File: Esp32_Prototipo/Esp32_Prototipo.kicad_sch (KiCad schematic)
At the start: 18 parts, among them J1 Fan, J2 Screw_Terminal_01x04, J3 Screw_Terminal_01x04, J4 Input, Q1 2N7002K, U1 ESP32-DEVKITC-32D

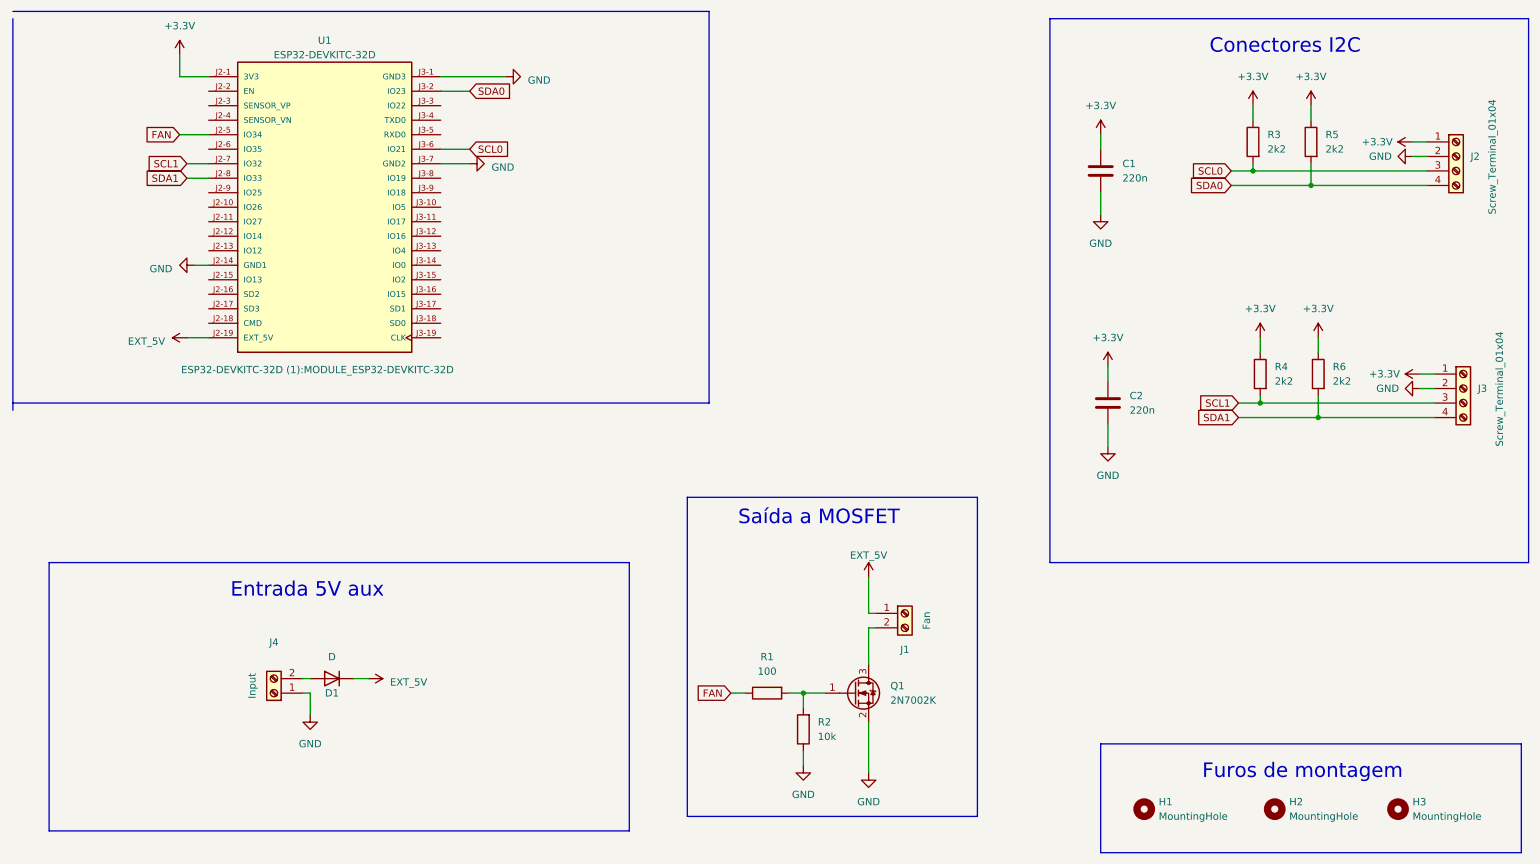
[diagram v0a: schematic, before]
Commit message: proto esp32 pronto para montar
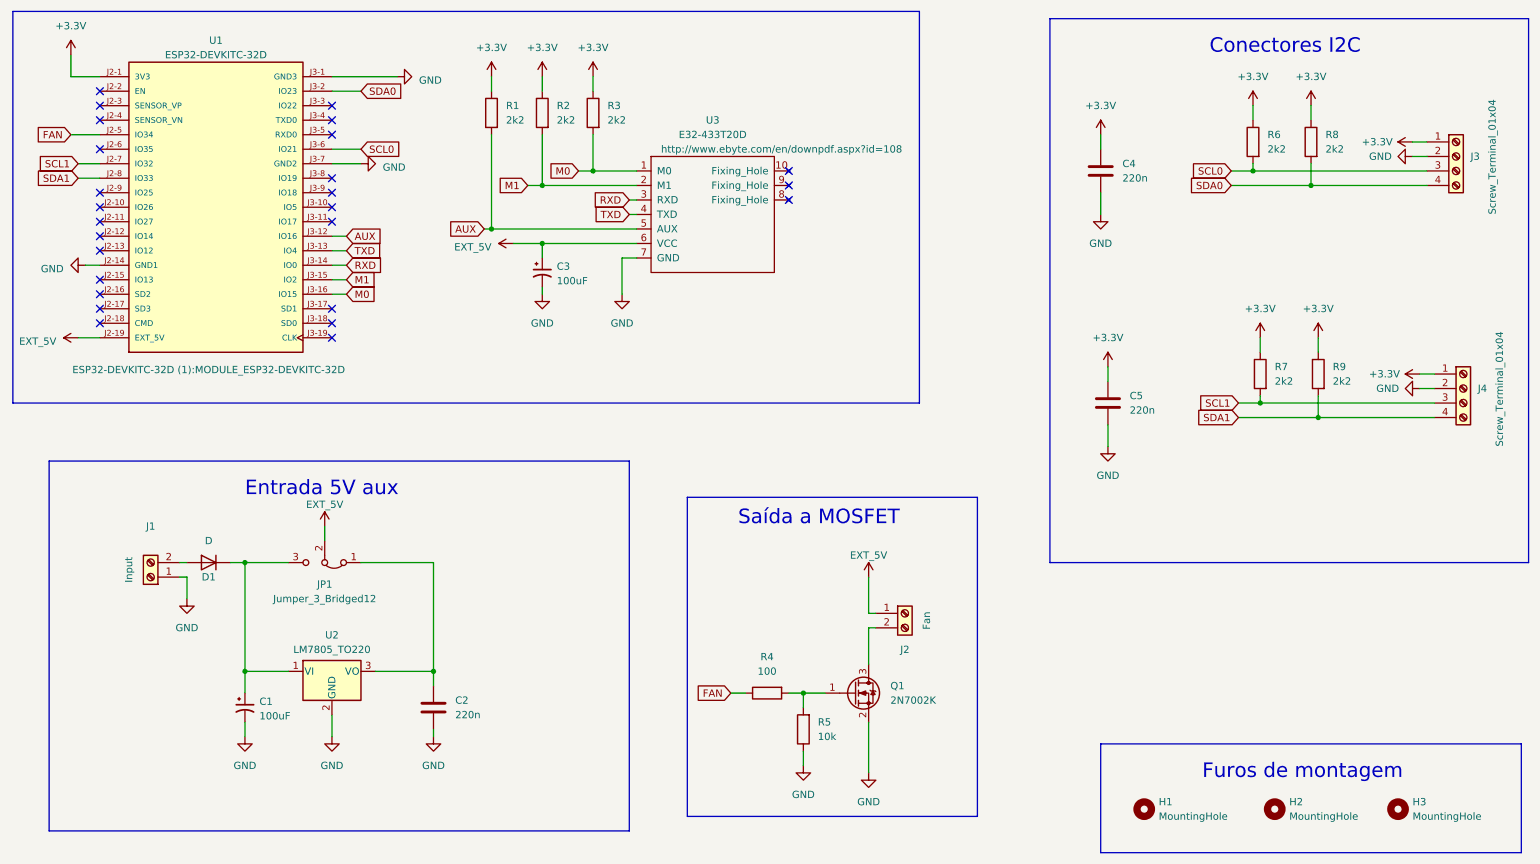
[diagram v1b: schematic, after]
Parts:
- added C1, C3: 100uF, Capacitor_THT:CP_Radial_D6.3mm_P2.50mm, symbol Device:C_Polarized_Small_US
- added C2: 220n, Capacitor_THT:C_Disc_D5.0mm_W2.5mm_P5.00mm, symbol Device:C
- added JP1: Jumper_3_Bridged12, Connector_PinHeader_2.54mm:PinHeader_1x03_P2.54mm_Vertical, symbol Jumper:Jumper_3_Bridged12
- added R1, R2, R3: 2k2, Resistor_THT:R_Axial_DIN0207_L6.3mm_D2.5mm_P10.16mm_Horizontal, symbol Device:R
- added U2: LM7805_TO220, Package_TO_SOT_THT:TO-220-3_Vertical, symbol Regulator_Linear:LM7805_TO220
- added U3: E32-433T20D, footprints6:E32-xxxT20D, symbol E32-xxxT20D:E32-433T20D
- renumbered C1 to C4, C2 to C5, J4 to J1, J1 to J2, J2 to J3, J3 to J4, R1 to R4, R2 to R5, R3 to R6, R4 to R7, R5 to R8, R6 to R9
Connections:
- net +3V3: now also R1.1, R2.1, R3.1
- net +BATT: now also C3.1, JP1.2 (C), U3.6 (VCC); no longer D1.1 (K)
- net GND: now also C1.2, C2.1, C3.2, U2.2 (GND), U3.7 (GND)
- net AUX: now reaches U1.J3-12 (IO16)
- net AUX: now also R1.2, U3.5 (AUX)
- net TXD: now reaches U1.J3-13 (IO4)
- net TXD: now also U3.4 (TXD)
- net RXD: now reaches U1.J3-14 (IO0)
- net RXD: now also U3.3 (RXD)
- net M1: now reaches U1.J3-15 (IO2)
- net M1: now also R2.2, U3.2 (M1)
- net M0: now reaches U1.J3-16 (IO15)
- net M0: now also R3.2, U3.1 (M0)
- new net: C1.1, D1.1 (K), JP1.3 (B), U2.1 (VI)
- new net: C2.2, JP1.1 (A), U2.3 (VO)
- no-connect marks 0 -> 26
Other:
- moved on the sheet: D1, J1, U1
